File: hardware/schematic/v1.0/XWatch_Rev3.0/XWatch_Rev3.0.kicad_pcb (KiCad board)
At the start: 2 copper layers, 36 x 36 mm, 158 parts, among them CN1 SCTA1A0100, CN2 SCTA1A0100, CN3 SCTA1A0100, CN4 SCTA1A0100, CN5 SCTA1A0100, CN6 SCTA1A0100, IC1 nRF52833-QDAA-R, U10 OPT3001DNPR, U11 MAX30101EFD_T, U12 DRV2605LDGSR, U13 SK6018D4-33, U14 AXE530127-DO0143FMST02, U15 STM32U5A9BJY6QTR, U16 R832000033-32MHZ, U2 GD25LQ128EWIGR, U3 DA9168, U4 TPS62840DLCR, U5 MAX17048G_T10, U6 LSM6DSOXTR, U7 LIS2MDLTR, U8 SM03B-SRSS-TB_LF_SN_P, U9 LPS27HHWTR, X1 32.768KHZ, X2 16MHZ, X3 32.768KHZ

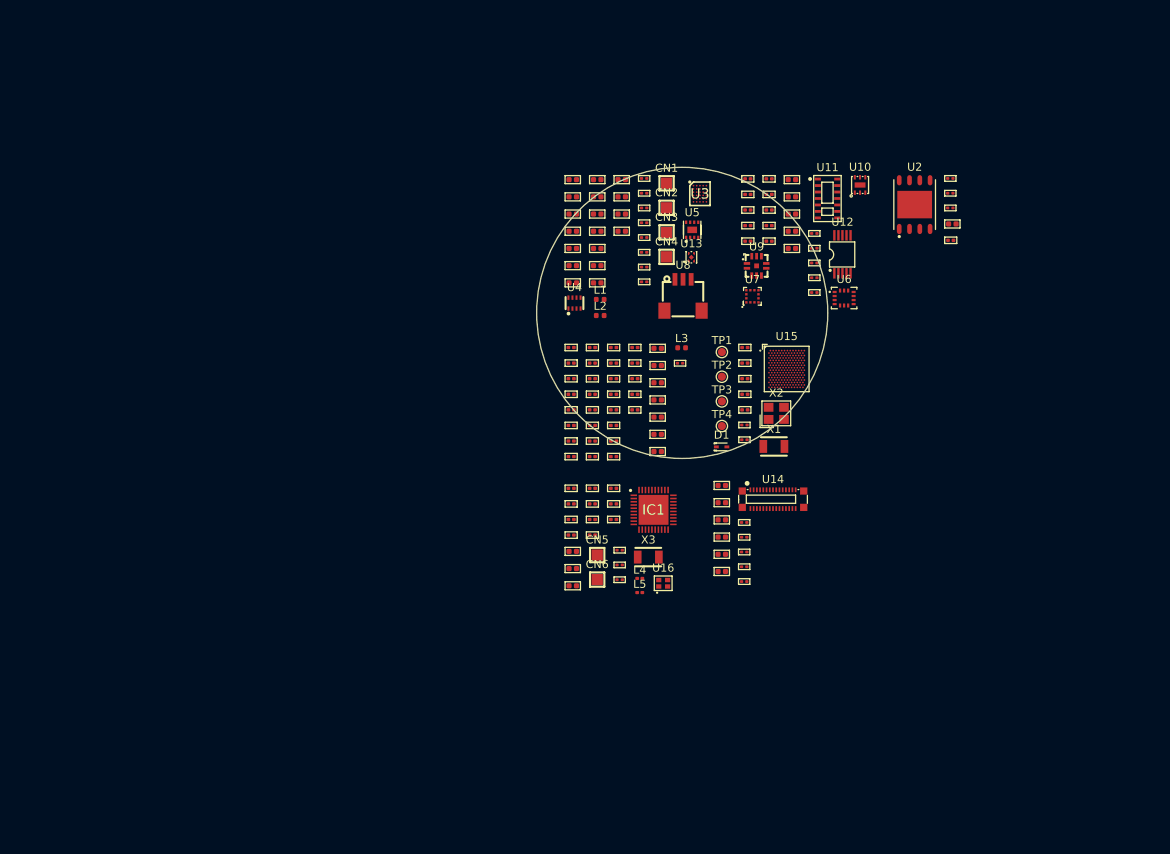
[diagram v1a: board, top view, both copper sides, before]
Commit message: add pdf
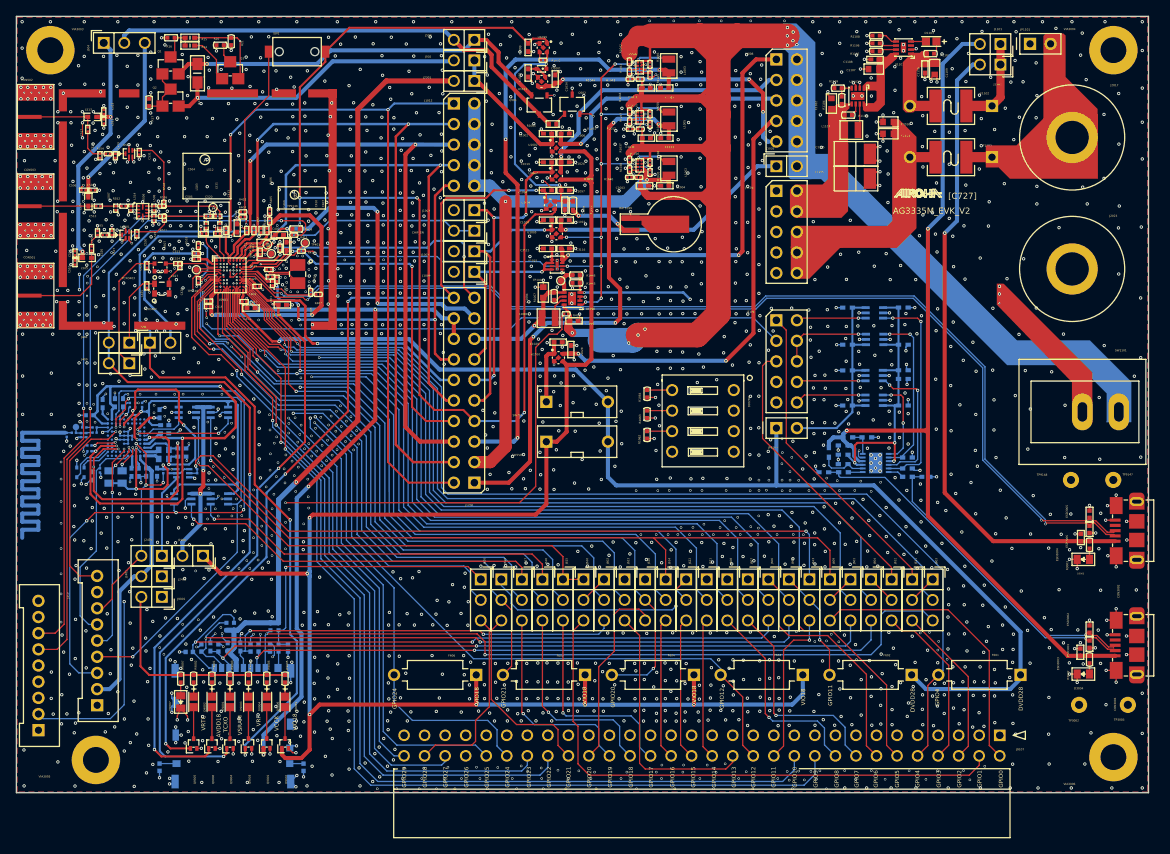
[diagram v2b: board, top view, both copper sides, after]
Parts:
- removed C1, C2, C86, C87: 5.6pF, XWatch_Rev3.0:GEN_C_0201
- removed C10, C109, C16, C17, C30, C59, C6, C63, C78, C9: 10uF, XWatch_Rev3.0:GEN_C_0402
- removed C100, C103, C106, C107, C108, C110, C111, C112, C113, C20, C21, C22, C23, C24, C25, C26, C27, C28, C29, C48, C50, C51, C53, C54, C55, C56, C57, C58, C60, C67, C69, C70, C72, C79, C89, C90, C91, C92, C93, C94, C95, C96, C97, C98: 100nF, XWatch_Rev3.0:GEN_C_0201
- removed C101, C102, C18, C19, C61, C62, C64, C65, C66, C68, C74, C76, C80, C81: 1uF, XWatch_Rev3.0:GEN_C_0402
- removed C104, C105, C11, C12, C13: 2.2uF, XWatch_Rev3.0:GEN_C_0402
- removed C14, C49, C7, C73, C75, C77: 100nF, XWatch_Rev3.0:GEN_C_0402
- removed C15, C5, C71, C99: 4.7uF, XWatch_Rev3.0:GEN_C_0402
- removed C3, C4: 10pF, XWatch_Rev3.0:GEN_C_0201
- removed C52: 220nF, XWatch_Rev3.0:GEN_C_0201
- removed C8: 47nF, XWatch_Rev3.0:GEN_C_0402
- removed C82: 1pF, XWatch_Rev3.0:GEN_C_0201
- removed C83: 1.2pF, XWatch_Rev3.0:GEN_C_0201
- removed C84, C85: 12pF, XWatch_Rev3.0:GEN_C_0201
- removed C88: 100pF, XWatch_Rev3.0:GEN_C_0201
- removed CN1, CN2, CN3, CN4, CN5, CN6: SCTA1A0100, XWatch_Rev3.0:SCTA1A0100
- removed D1: RB520S-30, XWatch_Rev3.0:RB520S-30_C7502701
- removed IC1: nRF52833-QDAA-R, XWatch_Rev3.0:QFN40P500X500X90-41N
- removed L1, L2, L3: 2.2uH, XWatch_Rev3.0:L_0402_1005Metric
- removed L4: 4.7nH, XWatch_Rev3.0:L_0201_0603Metric
- removed L5: 2.2nH, XWatch_Rev3.0:L_0201_0603Metric
- removed R10: 38.3 k 1%, XWatch_Rev3.0:GEN_R_0201
- removed R11, R12: 2.2K, XWatch_Rev3.0:GEN_R_0201
- removed R18, R23, R24, R25, R6, R7, R8: 10K, XWatch_Rev3.0:GEN_R_0201
- removed R19, R26, R27, R28, R3: 100K, XWatch_Rev3.0:GEN_R_0201
- removed R22, R29: 0, XWatch_Rev3.0:GEN_R_0201
- removed R4, R5: 4.7K, XWatch_Rev3.0:GEN_R_0201
- removed R9: 24.9 k 1%, XWatch_Rev3.0:GEN_R_0201
- removed TP1, TP2, TP3, TP4: TestPoint, TestPoint:TestPoint_Pad_D1.0mm
- removed U10: OPT3001DNPR, XWatch_Rev3.0:OPT3001DNPR
- removed U11: MAX30101EFD_T, XWatch_Rev3.0:MAX30101EFD_T
- removed U12: DRV2605LDGSR, XWatch_Rev3.0:DRV2605LDGSR
- removed U13: SK6018D4-33, XWatch_Rev3.0:SK6018D4-33
- removed U14: AXE530127-DO0143FMST02, XWatch_Rev3.0:AXE530127
- removed U15: STM32U5A9BJY6QTR, XWatch_Rev3.0:STM32U5A9BJY6QTR
- removed U16: R832000033-32MHZ, XWatch_Rev3.0:R832000033
- removed U2: GD25LQ128EWIGR, XWatch_Rev3.0:GD25LQ128EWIGR
- removed U3: DA9168, XWatch_Rev3.0:BGA30C40P5X6_214X254X56
- removed U4: TPS62840DLCR, XWatch_Rev3.0:TPS62840DLCR
- removed U5: MAX17048G_T10, XWatch_Rev3.0:MAX17048G_T10
- removed U6: LSM6DSOXTR, XWatch_Rev3.0:LSM6DSOXTR
- removed U7: LIS2MDLTR, XWatch_Rev3.0:LIS2MDLTR
- removed U8: SM03B-SRSS-TB_LF_SN_P, XWatch_Rev3.0:SM03B-SRSS-TB_LF_SN_P
- removed U9: LPS27HHWTR, XWatch_Rev3.0:LPS27HHWTR
- removed X1, X3: 32.768KHZ, XWatch_Rev3.0:NX3215SA_32_768KHZ_EXS00A-MU00525
- removed X2: 16MHZ, XWatch_Rev3.0:TXM16M0004252CBCEO00T
- added BAT1099: C0.22F3.3V$2F$SMD$2F$EN-RL, C0.22F3.3V$2F$SMD$2F$EN-RL, F.Cu at (154.7, 82.7)
- added C0401: C0201, C0201, F.Cu at (110.7, 89.5)
- added C0501: C0201, C0201, F.Cu at (87.8, 85.7)
- added C1002: C0402, C0402, F.Cu at (144.2, 71.5)
- added C1003: C0402, C0402, F.Cu at (156.2, 78.0)
- added C1004: C0402, C0402, F.Cu at (158.7, 78.0)
- added C1006: C0402, C0402, F.Cu at (146.4, 71.5)
- added C1014: C0402, C0402, F.Cu at (144.2, 82.2)
- added C1015: C0402, C0402, F.Cu at (146.4, 82.2)
- added C1019: C0402, C0402, F.Cu at (144.2, 75.0)
- added C1021: C0402, C0402, F.Cu at (156.4, 65.9)
- added C1022: C0402, C0402, F.Cu at (158.7, 65.9)
- added C1024: C0402, C0402, F.Cu at (146.4, 75.0)
- added C1025: C0402, C0402, F.Cu at (145.5, 97.3)
- added C1028: C0402, C0402, F.Cu at (147.1, 98.2)
- added C1030: C0402, C0402, F.Cu at (156.4, 72.1)
- added C1031: C0402, C0402, F.Cu at (158.7, 72.1)
- added C1034: C0402, C0402, F.Cu at (145.1, 64.7)
- added C1035: C0402, C0402, F.Cu at (141.8, 64.0)
- added C1094: C0603, C0603, F.Cu at (143.7, 91.1)
- added C1095: C0402, C0402, F.Cu at (147.5, 94.7)
- added C1096: C0402, C0402, F.Cu at (144.2, 78.5)
- added C1097: C0402, C0402, F.Cu at (146.4, 78.5)
- added C1098: C0402, C0402, F.Cu at (146.3, 80.4)
- added C1099: C0402, C0402, F.Cu at (141.8, 60.8)
- added C1102: C0603, C0603, F.Cu at (179.3, 67.8)
- added C1104: C0603, C0603, F.Cu at (186.3, 71.5)
- added C1105: C1210, C1210, F.Cu at (182.3, 74.0)
- added C1106: C1210, C1210, F.Cu at (182.3, 77.1)
- added C1107: C0603, C0603, F.Cu at (184.5, 63.5)
- added C1108: C0402, C0402, F.Cu at (184.7, 62.3)
- added C1109: C0603, C0603, F.Cu at (192.1, 63.5)
- added C1110: C0402, C0402, F.Cu at (190.8, 63.5)
- added C2016: C0603, C0603, F.Cu at (186.3, 70.1)
- added C2301: C0402, C0402, B.Cu at (104.6, 135.0)
- added C2302: C0402, C0402, B.Cu at (106.2, 135.0)
- added C2303: C0402, C0402, B.Cu at (102.5, 135.0)
- added C2401: C0201, C0201, B.Cu at (87.2, 108.8)
- added C2402: C0402, C0402, B.Cu at (99.0, 110.4)
- added C2403: C0402, C0402, B.Cu at (96.8, 107.6)
- added C2404: C0402, C0402, B.Cu at (96.8, 108.6)
- added C2405: C0201, C0201, B.Cu at (87.5, 110.1)
- added C2406: C0201, C0201, B.Cu at (87.5, 110.8)
- added C2407: C0402, C0402, B.Cu at (95.9, 113.4)
- added C2408: C0201, C0201, B.Cu at (84.7, 108.7)
- added C2409: C0201, C0201, B.Cu at (86.5, 108.8)
- added C2410: C0201, C0201, B.Cu at (86.9, 107.8)
- added C2411: C0402, C0402, B.Cu at (87.9, 113.8)
- added C2412: C0402, C0402, B.Cu at (94.6, 113.4)
- added C2413: C0402, C0402, B.Cu at (99.0, 111.4)
- added C2414: C0402, C0402, B.Cu at (93.6, 113.4)
- added C2415: C0402, C0402, B.Cu at (96.2, 106.1)
- added C2416: C0402, C0402, B.Cu at (92.7, 113.4)
- added C2417: C0402, C0402, B.Cu at (87.5, 106.3)
- added C2418: C0201, C0201, B.Cu at (93.2, 105.1)
- added C2419: C0402, C0402, B.Cu at (89.2, 104.9)
- added C2420: C0402, C0402, B.Cu at (90.7, 104.8)
- added C2421: C0201, C0201, B.Cu at (94.0, 105.1)
- added C3101: SC0402, SC0402, B.Cu at (180.7, 112.4)
- added C3102: C0402, C0402, B.Cu at (191.0, 113.9)
- added C3103: SC0402, SC0402, B.Cu at (188.2, 100.8)
- added C3104: SC0402, SC0402, B.Cu at (181.3, 100.8)
- added C3105: SC0402, SC0402, B.Cu at (178.3, 113.4)
- added C3106: SC0402, SC0402, B.Cu at (188.2, 97.6)
- added C3107: SC0402, SC0402, B.Cu at (180.7, 110.1)
- added C3108: SC0402, SC0402, B.Cu at (180.7, 111.2)
- added C3109: SC0402, SC0402, B.Cu at (188.2, 93.0)
- added C3110: SC0402, SC0402, B.Cu at (181.3, 93.0)
- added C3111: SC0402, SC0402, B.Cu at (188.2, 105.1)
- added C3112: SC0402, SC0402, B.Cu at (181.3, 97.6)
- added C3113: SC0402, SC0402, B.Cu at (188.2, 101.8)
- added C3114: SC0402, SC0402, B.Cu at (181.3, 105.1)
- added C3115: C0402, C0402, F.Cu at (144.2, 85.7)
- added C3116: C0402, C0402, F.Cu at (146.4, 85.7)
- added C402: C0201, C0201, F.Cu at (108.8, 83.5)
- added C403: C0201, C0201, F.Cu at (109.5, 83.5)
- added C404: C0402, C0402, F.Cu at (105.8, 83.2)
- added C405: C0402, C0402, F.Cu at (111.0, 84.0)
- added C406: C0402, C0402, F.Cu at (111.4, 92.7)
- added C407: C0201, C0201, F.Cu at (111.1, 85.7)
- added C408: C0201, C0201, F.Cu at (108.3, 90.4)
- added C409: C0201, C0201, F.Cu at (108.7, 86.2)
- added C410: C0402, C0402, F.Cu at (111.9, 85.4)
- added C411: C0201, C0201, F.Cu at (107.0, 83.5)
- added C412: C0201, C0201, F.Cu at (107.9, 83.5)
- added C413: C0201, C0201, F.Cu at (104.4, 83.5)
- added C414: C0402, C0402, F.Cu at (107.5, 93.1)
- added C415: C0201, C0201, F.Cu at (102.3, 92.9)
- added C416: C0201, C0201, F.Cu at (102.3, 92.2)
- added C417: C0201, C0201, F.Cu at (106.7, 92.3)
- added C419: C0201, C0201, F.Cu at (109.7, 88.3)
- added C420: C0201, C0201, F.Cu at (109.9, 89.2)
- added C425: C0201, C0201, F.Cu at (94.6, 90.3)
- added C426: C0201, C0201, F.Cu at (98.7, 87.8)
- added C427: C0201, C0201, F.Cu at (98.5, 87.6)
- added C428: C0201, C0201, F.Cu at (94.6, 87.8)
- added C504: C0201, C0201, F.Cu at (102.2, 81.7)
- added C505: C0201, C0201, F.Cu at (101.7, 83.9)
- added C506: C0201, C0201, F.Cu at (86.8, 78.5)
- added C508: C0201, C0201, F.Cu at (88.0, 78.5)
- added C510: C0201, C0201, F.Cu at (85.7, 87.5)
- added C511: C0201, C0201, F.Cu at (85.7, 86.3)
- added C513: C0201, C0201, F.Cu at (88.6, 80.5)
- added C517: C0201, C0201, F.Cu at (87.3, 71.0)
- added C520: C0201, C0201, F.Cu at (103.4, 83.9)
- added C521: C0201, C0201, F.Cu at (89.3, 70.0)
- added C522: C0201, C0201, F.Cu at (89.3, 68.8)
- added C523: C0201, C0201, F.Cu at (100.8, 86.3)
- added C524: C0201, C0201, F.Cu at (100.8, 87.0)
- added C525: C0201, C0201, F.Cu at (101.0, 89.7)
- added C526: C0201, C0201, F.Cu at (88.5, 83.8)
- added C527: C0201, C0201, F.Cu at (90.3, 83.8)
- added C528: C0201, C0201, F.Cu at (88.8, 74.2)
- added C529: C0201, C0201, F.Cu at (90.7, 74.2)
- added C530: C0201, C0201, F.Cu at (93.4, 83.9)
- added C531: C0201, C0201, F.Cu at (93.7, 73.8)
- added CHIP_EN: DIP2$2F$P2.54, DIP2$2F$P2.54, F.Cu at (135.1, 83.5)
- added CON2301: MICROSD$2F$8P$2F$SMD$2F$TA-M017-012-07-811, MICROSD$2F$8P$2F$SMD$2F$TA-M017-012-07-811, B.Cu at (103.0, 137.1)
- added CON3001: MICROUSB$2F$5P$2F$SMD$2F$P0.65$2F$R$2F$8791-N005-M1A0, MICROUSB$2F$5P$2F$SMD$2F$P0.65$2F$R$2F$8791-N005-M1A0, F.Cu at (214.4, 134.8)
- added CON3002: MICROUSB$2F$5P$2F$SMD$2F$P0.65$2F$R$2F$8791-N005-M1A0, MICROUSB$2F$5P$2F$SMD$2F$P0.65$2F$R$2F$8791-N005-M1A0, F.Cu at (214.4, 120.6)
- added CON501: SMA8400M, SMA8400M, F.Cu at (80.1, 91.5)
- added CON502: SMA8400M, SMA8400M, F.Cu at (80.1, 69.4)
- added CON503: SMA8400M, SMA8400M, F.Cu at (80.1, 80.5)
- added D1001: D$2F$SMD$2F$VMD2, D$2F$SMD$2F$VMD2, F.Cu at (143.4, 63.5)
- added D1103: LED190, LED190, F.Cu at (191.6, 60.1)
- added D2401: LED-S, LED-S, B.Cu at (91.6, 114.0)
- added D2402: LED-S, LED-S, B.Cu at (90.0, 114.0)
- added D3004: LED-S, LED-S, F.Cu at (210.4, 138.3)
- added D3005: LED-S, LED-S, F.Cu at (210.4, 124.1)
- added D9001: LED190, LED190, F.Cu at (102.7, 141.8)
- added D9002: LED190, LED190, F.Cu at (100.4, 141.8)
- added D9003: LED190, LED190, F.Cu at (104.9, 141.8)
- added D9004: LED190, LED190, F.Cu at (107.2, 141.8)
- added D9005: LED190, LED190, F.Cu at (111.7, 141.8)
- added D9006: LED190, LED190, F.Cu at (109.5, 141.8)
- added D9007: LED-S, LED-S, F.Cu at (98.8, 141.8)
- added ESD2301: VR0402, VR0402, B.Cu at (112.1, 135.1)
- added ESD2302: VR0402, VR0402, B.Cu at (109.9, 135.1)
- added ESD2303: VR0402, VR0402, B.Cu at (108.4, 135.1)
- added ESD2304: VR0402, VR0402, B.Cu at (107.5, 135.1)
- added ESD2305: VR0402, VR0402, B.Cu at (103.5, 135.1)
- added ESD2306: VR0402, VR0402, B.Cu at (101.4, 135.1)
- added ESD2307: VR0402, VR0402, B.Cu at (99.9, 135.6)
- added ESD2308: VR0402, VR0402, B.Cu at (114.0, 149.9)
- added ESD239: VR0402, VR0402, B.Cu at (96.2, 149.9)
- added ESD3001: VR0402, VR0402, F.Cu at (211.2, 134.6)
- added ESD3002: VR0402, VR0402, F.Cu at (211.2, 132.8)
- added ESD3003: VR0402, VR0402, F.Cu at (210.1, 135.6)
- added ESD3004: VR0402, VR0402, F.Cu at (210.1, 121.5)
- added ESD3005: VR0402, VR0402, F.Cu at (211.2, 118.6)
- added ESD3006: VR0402, VR0402, F.Cu at (211.2, 120.4)
- added F1102: FUSE$2F$DIP$2F$SMD, FUSE$2F$DIP$2F$SMD, F.Cu at (199.2, 68.1)
- added F1103: FUSE$2F$DIP$2F$SMD, FUSE$2F$DIP$2F$SMD, F.Cu at (199.2, 74.4)
- added F601: R$5C$DIP, R$5C$DIP, F.Cu at (197.6, 138.4)
- added F602: R$5C$DIP, R$5C$DIP, F.Cu at (184.1, 138.4)
- added F603: R$5C$DIP, R$5C$DIP, F.Cu at (170.7, 138.4)
- added F604: R$5C$DIP, R$5C$DIP, F.Cu at (157.2, 138.4)
- added F605: R$5C$DIP, R$5C$DIP, F.Cu at (143.7, 138.4)
- added F606: R$5C$DIP, R$5C$DIP, F.Cu at (130.3, 138.4)
- added J1002: DIP2$2F$P2.54, DIP2$2F$P2.54, F.Cu at (135.1, 81.0)
- added J1005: DIP2$2F$P2.54, DIP2$2F$P2.54, F.Cu at (172.5, 75.5)
- added J1007: DIP2$2F$P2.54, DIP2$2F$P2.54, F.Cu at (135.1, 86.1)
- added J1008: HEADER10, HEADER10, F.Cu at (172.5, 62.3)
- added J1009: DIP2$2F$P2.54, DIP2$2F$P2.54, F.Cu at (135.1, 88.6)
- added J1012: HEADER10, HEADER10, F.Cu at (132.6, 67.8)
- added J1101: DIP2$2F$P2.54, DIP2$2F$P2.54, F.Cu at (200.2, 60.4)
- added J1102: DIP2$2F$P2.54, DIP2$2F$P2.54, F.Cu at (200.2, 63.0)
- added J1103: HEADER10, HEADER10, F.Cu at (172.5, 78.6)
- added J1206: HEADER10X2-P2.54, HEADER10X2-P2.54, F.Cu at (132.6, 91.8)
- added J2017: JACK$2F$BANAAA, JACK$2F$BANAAA, F.Cu at (209.1, 72.0)
- added J2023: JACK$2F$BANAAA, JACK$2F$BANAAA, F.Cu at (209.1, 88.2)
- added J2301: DIP2$2F$P2.54, DIP2$2F$P2.54, F.Cu at (135.1, 65.0)
- added J2401: SIP-9P-2MM-FRAME, SIP-9P-2MM-FRAME, F.Cu at (88.5, 134.2)
- added J2402: DIP2$2F$P2.54, DIP2$2F$P2.54, F.Cu at (96.5, 126.3)
- added J2403: DIP2$2F$P2.54, DIP2$2F$P2.54, F.Cu at (96.5, 123.7)
- added J3101: HEADER10, HEADER10, F.Cu at (172.5, 94.6)
- added J408: DIP2$2F$P2.54, DIP2$2F$P2.54, F.Cu at (92.5, 97.4)
- added J409: DIP2$2F$P2.54, DIP2$2F$P2.54, F.Cu at (92.5, 99.9)
- added J412: SIP-9P-2MM-FRAME, SIP-9P-2MM-FRAME, F.Cu at (81.2, 137.3)
- added J501: DIP2$2F$P2.54, DIP2$2F$P2.54, F.Cu at (95.0, 97.4)
- added J502: DIP2$2F$P2.54, DIP2$2F$P2.54, F.Cu at (135.1, 62.4)
- added J503: DIP2$2F$P2.54, DIP2$2F$P2.54, F.Cu at (135.1, 59.9)
- added J504: DIP3$2F$P2.54, DIP3$2F$P2.54, F.Cu at (89.3, 60.3)
- added J601: DIP3$2F$P2.54, DIP3$2F$P2.54, F.Cu at (181.7, 126.6)
- added J602: DIP3$2F$P2.54, DIP3$2F$P2.54, F.Cu at (151.2, 126.6)
- added J603: DIP3$2F$P2.54, DIP3$2F$P2.54, F.Cu at (191.8, 126.6)
- added J604: DIP3$2F$P2.54, DIP3$2F$P2.54, F.Cu at (184.2, 126.6)
- added J605: DIP3$2F$P2.54, DIP3$2F$P2.54, F.Cu at (174.0, 126.6)
- added J606: DIP3$2F$P2.54, DIP3$2F$P2.54, F.Cu at (171.5, 126.6)
- added J607: DIP3$2F$P2.54, DIP3$2F$P2.54, F.Cu at (169.0, 126.6)
- added J608: DIP3$2F$P2.54, DIP3$2F$P2.54, F.Cu at (166.4, 126.6)
- added J609: DIP3$2F$P2.54, DIP3$2F$P2.54, F.Cu at (179.1, 126.6)
- added J610: DIP3$2F$P2.54, DIP3$2F$P2.54, F.Cu at (148.6, 126.6)
- added J611: DIP3$2F$P2.54, DIP3$2F$P2.54, F.Cu at (189.3, 126.6)
- added J612: DIP3$2F$P2.54, DIP3$2F$P2.54, F.Cu at (186.7, 126.6)
- added J613: DIP3$2F$P2.54, DIP3$2F$P2.54, F.Cu at (176.6, 126.6)
- added J614: DIP3$2F$P2.54, DIP3$2F$P2.54, F.Cu at (158.8, 126.6)
- added J615: DIP3$2F$P2.54, DIP3$2F$P2.54, F.Cu at (146.1, 126.6)
- added J616: DIP3$2F$P2.54, DIP3$2F$P2.54, F.Cu at (143.6, 126.6)
- added J617: DIP3$2F$P2.54, DIP3$2F$P2.54, F.Cu at (141.0, 126.6)
- added J618: DIP3$2F$P2.54, DIP3$2F$P2.54, F.Cu at (156.3, 126.6)
- added J619: DIP3$2F$P2.54, DIP3$2F$P2.54, F.Cu at (138.5, 126.6)
- added J620: DIP3$2F$P2.54, DIP3$2F$P2.54, F.Cu at (135.9, 126.6)
- added J621: DIP3$2F$P2.54, DIP3$2F$P2.54, F.Cu at (163.9, 126.6)
- added J622: DIP3$2F$P2.54, DIP3$2F$P2.54, F.Cu at (161.3, 126.6)
- added J623: DIP3$2F$P2.54, DIP3$2F$P2.54, F.Cu at (153.7, 126.6)
- added J9001: DIP2$2F$P2.54, DIP2$2F$P2.54, F.Cu at (96.5, 128.8)
- added J9107: DIP30X2$2F$P2.54$2F$R$2F$PHR230GB138, DIP30X2$2F$P2.54$2F$R$2F$PHR230GB138, F.Cu at (200.1, 145.9)
- added J9109: DIP2$2F$P2.54, DIP2$2F$P2.54, F.Cu at (101.6, 123.7)
- added JP1101: SIP-2P, SIP-2P, F.Cu at (203.9, 60.4)
- added JP3103: SIP-2P, SIP-2P, F.Cu at (172.5, 107.9)
- added L1001: L$2F$IND$2F$SMD$2F$2520, L$2F$IND$2F$SMD$2F$2520, F.Cu at (144.3, 94.3)
- added L1002: L$2F$IND$2F$SMD$2F$LQM2MP-0806, L$2F$IND$2F$SMD$2F$LQM2MP-0806, F.Cu at (159.2, 75.8)
- added L1003: L$2F$IND$2F$SMD$2F$LQM2MP-0806, L$2F$IND$2F$SMD$2F$LQM2MP-0806, F.Cu at (159.2, 63.1)
- added L1005: L$2F$IND$2F$SMD$2F$LQM2MP-0806, L$2F$IND$2F$SMD$2F$LQM2MP-0806, F.Cu at (159.2, 69.7)
- added L1102: L$2F$IND$2F$SMD$2F$2520, L$2F$IND$2F$SMD$2F$2520, F.Cu at (181.8, 71.1)
- added L2401: C0201, C0201, B.Cu at (88.2, 108.5)
- added L2402: C0603_H300, C0603_H300, B.Cu at (96.7, 110.8)
- added L2403: C0201, C0201, B.Cu at (88.2, 107.8)
- added L2404: C0603_H300, C0603_H300, B.Cu at (96.7, 111.9)
- added L401: L0201, L0201, F.Cu at (110.2, 90.0)
- added L503: L0201, L0201, F.Cu at (102.0, 82.9)
- added L504: L$2F$IND$2F$SMD$2F$0402, L$2F$IND$2F$SMD$2F$0402, F.Cu at (87.4, 79.9)
- added L505: L$2F$IND$2F$SMD$2F$0402, L$2F$IND$2F$SMD$2F$0402, F.Cu at (87.2, 86.9)
- added L507: L0201, L0201, F.Cu at (90.8, 80.7)
- added L508: L0201, L0201, F.Cu at (95.5, 80.7)
- added L511: L0201, L0201, F.Cu at (103.7, 82.9)
- added L512: L0201, L0201, F.Cu at (103.4, 81.7)
- added L513: L$2F$IND$2F$SMD$2F$0402, L$2F$IND$2F$SMD$2F$0402, F.Cu at (87.9, 69.4)
- added L514: L0201, L0201, F.Cu at (92.7, 80.7)
- added L515: L0201, L0201, F.Cu at (95.5, 82.0)
- added PF_TEST2401: PADCB, PADCB, B.Cu at (85.6, 107.8)
- added Q1: SOT-23, SOT-23, F.Cu at (96.6, 64.1)
- added Q2: SOT-23, SOT-23, F.Cu at (96.6, 68.1)
- added Q3: SOT-23, SOT-23, F.Cu at (103.9, 64.7)
- added Q501: SPP2301_USI, SPP2301_USI, F.Cu at (143.2, 68.0)
- added Q502: SPP2301_USI, SPP2301_USI, F.Cu at (147.2, 67.9)
- added Q9001: 2-1L1B$2F$SMD$2F$SSM3K35MFV, 2-1L1B$2F$SMD$2F$SSM3K35MFV, F.Cu at (109.5, 146.9)
- added Q9002: 2-1L1B$2F$SMD$2F$SSM3K35MFV, 2-1L1B$2F$SMD$2F$SSM3K35MFV, F.Cu at (111.7, 146.9)
- added Q9003: 2-1L1B$2F$SMD$2F$SSM3K35MFV, 2-1L1B$2F$SMD$2F$SSM3K35MFV, F.Cu at (107.2, 146.9)
- added Q9004: 2-1L1B$2F$SMD$2F$SSM3K35MFV, 2-1L1B$2F$SMD$2F$SSM3K35MFV, F.Cu at (104.9, 146.9)
- added Q9005: 2-1L1B$2F$SMD$2F$SSM3K35MFV, 2-1L1B$2F$SMD$2F$SSM3K35MFV, F.Cu at (100.4, 146.9)
- added Q9006: 2-1L1B$2F$SMD$2F$SSM3K35MFV, 2-1L1B$2F$SMD$2F$SSM3K35MFV, F.Cu at (102.7, 146.9)
- added R1033: R0201, R0201, F.Cu at (143.6, 62.4)
- added R1035: R0201, R0201, F.Cu at (156.9, 76.3)
- added R1036: R0201, R0201, F.Cu at (156.9, 75.1)
- added R1037: R0201, R0201, F.Cu at (154.3, 74.8)
- added R1038: R0201, R0201, F.Cu at (154.3, 76.0)
- added R1039: R0201, R0201, F.Cu at (154.3, 76.9)
- added R1040: R0201, R0201, F.Cu at (155.5, 76.9)
- added R1041: R0201, R0201, F.Cu at (154.3, 63.9)
- added R1042: R0201, R0201, F.Cu at (154.3, 62.6)
- added R1043: R0201, R0201, F.Cu at (155.6, 64.8)
- added R1044: R0201, R0201, F.Cu at (154.4, 64.8)
- added R1045: R0201, R0201, F.Cu at (156.9, 64.3)
- added R1046: R0201, R0201, F.Cu at (156.9, 62.9)
- added R1047: R0201, R0201, F.Cu at (154.3, 70.0)
- added R1048: R0201, R0201, F.Cu at (154.3, 68.8)
- added R1049: R0201, R0201, F.Cu at (156.9, 70.4)
- added R1050: R0201, R0201, F.Cu at (156.9, 69.1)
- added R1051: R0201, R0201, F.Cu at (154.4, 70.9)
- added R1052: R0201, R0201, F.Cu at (155.6, 70.9)
- added R1060: R0402$2F$SMD, R0402$2F$SMD, F.Cu at (147.3, 80.4)
- added R1061: 0402_USI, 0402_USI, F.Cu at (144.8, 70.3)
- added R1062: R0402, R0402, F.Cu at (156.5, 108.8)
- added R1063: R0402, R0402, F.Cu at (156.5, 106.2)
- added R1064: R0402, R0402, F.Cu at (156.5, 103.7)
- added R1065: R0402, R0402, F.Cu at (147.7, 90.0)
- added R1067: R0402, R0402, F.Cu at (145.0, 91.6)
- added R1068: R0402, R0402, F.Cu at (147.7, 89.0)
- added R1103: R0402, R0402, F.Cu at (191.5, 61.6)
- added R1104: R0402, R0402, F.Cu at (180.6, 67.4)
- added R1105: R0402, R0402, F.Cu at (181.4, 69.2)
- added R1106: R0402, R0402, F.Cu at (184.8, 60.3)
- added R1107: R0402, R0402, F.Cu at (184.8, 61.3)
- added R1108: R0402, R0402, F.Cu at (184.8, 59.4)
- added R1109: R0402, R0402, F.Cu at (180.1, 65.9)
- added R2308: R0402, R0402, B.Cu at (109.9, 132.5)
- added R2309: R0402, R0402, B.Cu at (105.4, 132.5)
- added R2310: R0402, R0402, B.Cu at (104.5, 132.5)
- added R2311: R0402, R0402, B.Cu at (110.9, 132.5)
- added R2312: R0402, R0402, B.Cu at (110.9, 135.1)
- added R2401: R0201, R0201, B.Cu at (85.6, 108.5)
- added R2402: C0201, C0201, B.Cu at (92.5, 105.1)
- added R2403: C0402, C0402, B.Cu at (91.7, 104.8)
- added R2404: C0201, C0201, B.Cu at (88.8, 113.1)
- added R2405: R0201, R0201, B.Cu at (97.3, 113.2)
- added R2406: R0201, R0201, B.Cu at (96.7, 113.2)
- added R2409: R0201, R0201, B.Cu at (100.9, 113.2)
- added R3002: R0402, R0402, F.Cu at (211.2, 136.5)
- added R3003: R0402, R0402, F.Cu at (211.2, 122.4)
- added R3101: SR0402, SR0402, B.Cu at (179.0, 110.9)
- added R3102: SR0402, SR0402, B.Cu at (188.7, 113.9)
- added R3103: SR0402, SR0402, B.Cu at (181.3, 109.1)
- added R3104: SR0402, SR0402, B.Cu at (188.7, 112.9)
- added R3105: SR0402, SR0402, B.Cu at (180.8, 113.4)
- added R3106: SR0402, SR0402, B.Cu at (188.7, 111.6)
- added R3107: SR0402, SR0402, B.Cu at (183.7, 109.1)
- added R404: R0201, R0201, F.Cu at (106.5, 81.8)
- added R405: R0201, R0201, F.Cu at (109.8, 82.3)
- added R406: R0201, R0201, F.Cu at (109.8, 81.1)
- added R407: R0201, R0201, F.Cu at (115.8, 91.4)
- added R408: R0201, R0201, F.Cu at (114.9, 91.1)
- added R409: R0402, R0402, F.Cu at (113.1, 83.3)
- added R410: R0201, R0201, F.Cu at (146.5, 93.8)
- added R411: R0201, R0201, F.Cu at (112.8, 84.1)
- added R412: R0201, R0201, F.Cu at (106.5, 81.2)
- added R413: R0201, R0201, F.Cu at (113.7, 86.0)
- added R507: R0201, R0201, F.Cu at (96.8, 82.0)
- added R511: R0201, R0201, F.Cu at (96.5, 81.7)
- added R526: R0201, R0201, F.Cu at (96.5, 80.5)
- added R528: R0201, R0201, F.Cu at (96.7, 80.2)
- added R552: R0201, R0201, F.Cu at (91.8, 80.5)
- added R553: R0201, R0201, F.Cu at (101.0, 85.3)
- added R554: R0201, R0201, F.Cu at (89.8, 74.0)
- added R555: R0201, R0201, F.Cu at (89.4, 84.0)
- added R9001: R0402, R0402, F.Cu at (102.7, 138.9)
- added R9002: R0402, R0402, F.Cu at (100.4, 138.9)
- added R9003: R0402, R0402, F.Cu at (104.9, 138.9)
- added R9004: R0402, R0402, F.Cu at (107.2, 138.9)
- added R9005: R0402, R0402, F.Cu at (111.7, 138.9)
- added R9006: R0402, R0402, F.Cu at (109.5, 138.9)
- added R9007: R0402, R0402, F.Cu at (98.8, 138.9)
- added SHORT402: NC$2F$MMD$2F$L1$2F$4MIL, NC$2F$MMD$2F$L1$2F$4MIL, F.Cu at (108.8, 86.3)
- added SW1: TS6301E180G, TS6301E180G, F.Cu at (113.2, 61.4)
- added SW1101: SW2P$2F$DIP-V1, SW2P$2F$DIP-V1, F.Cu at (210.3, 105.9)
- added SW1V8: DIP-SWITCH_2X1, DIP-SWITCH_2X1, F.Cu at (144.0, 109.6)
- added SW2002: SW8P_DIP_P2.54, SW8P_DIP_P2.54, F.Cu at (163.4, 107.0)
- added SW2V8: DIP-SWITCH_2X1, DIP-SWITCH_2X1, F.Cu at (144.0, 104.7)
- added TCXO402: TXCO4P$2F$SMD$2F$P0.4$2F$2.0X1.6$2F$KT2016K, TXCO4P$2F$SMD$2F$P0.4$2F$2.0X1.6$2F$KT2016K, F.Cu at (96.5, 90.7)
- added TCXO403: TXCO4P$2F$SMD$2F$P0.4$2F$1.65X1.25$2F$1612TCXO, TXCO4P$2F$SMD$2F$P0.4$2F$1.65X1.25$2F$1612TCXO, F.Cu at (96.3, 88.0)
- added TP1001: TP30MIL, TP30MIL, F.Cu at (145.8, 89.7)
- added TP3002: HOLE$2F$PTH$2F$D1R2, HOLE$2F$PTH$2F$D1R2, F.Cu at (209.9, 142.1)
- added TP3003: HOLE$2F$PTH$2F$D1R2, HOLE$2F$PTH$2F$D1R2, F.Cu at (215.9, 142.1)
- added TP401: TP30MIL, TP30MIL, F.Cu at (114.2, 85.0)
- added TP9146: TP30MIL, TP30MIL, F.Cu at (110.0, 86.4)
- added TP9147: HOLE$2F$PTH$2F$D1R2, HOLE$2F$PTH$2F$D1R2, F.Cu at (214.1, 114.3)
- added TP9148: HOLE$2F$PTH$2F$D1R2, HOLE$2F$PTH$2F$D1R2, F.Cu at (208.9, 114.3)
- added TP9149: TP30MIL, TP30MIL, F.Cu at (100.8, 88.3)
- added U0401: AG3335M_3.8X4.2(R9XC10)-0.4BPAA, AG3335M_3.8X4.2(R9XC10)-0.4BPAA, F.Cu at (104.9, 89.0)
- added U0501: SAW-1.1X0.9, SAW-1.1X0.9, F.Cu at (92.0, 84.0)
- added U1002: ZQFN-4L-1X1, ZQFN-4L-1X1, F.Cu at (145.3, 73.3)
- added U1005: ZQFN-4L-1X1, ZQFN-4L-1X1, F.Cu at (145.3, 83.9)
- added U1007: ZQFN-4L-1X1, ZQFN-4L-1X1, F.Cu at (145.3, 76.7)
- added U1008: WL-CSP0.9X1.6-8, WL-CSP0.9X1.6-8, F.Cu at (155.6, 63.3)
- added U1010: ZQFN-4L-1X1, ZQFN-4L-1X1, F.Cu at (145.5, 99.2)
- added U1012: WL-CSP0.9X1.6-8, WL-CSP0.9X1.6-8, F.Cu at (155.6, 69.5)
- added U1014: ZQFN-4L-1X1, ZQFN-4L-1X1, F.Cu at (143.4, 65.1)
- added U1015: XDFN8-P0.4-1.6X1.2, XDFN8-P0.4-1.6X1.2, F.Cu at (145.4, 87.7)
- added U1016: WL-CSP0.9X1.6-8, WL-CSP0.9X1.6-8, F.Cu at (155.6, 75.4)
- added U1096: WDFN8$2F$SMD$2F$P0.5$2F$RT5715, WDFN8$2F$SMD$2F$P0.5$2F$RT5715, F.Cu at (147.2, 91.9)
- added U1098: ZQFN-4L-1X1, ZQFN-4L-1X1, F.Cu at (144.5, 80.3)
- added U1099: ZQFN-4L-1X1, ZQFN-4L-1X1, F.Cu at (143.7, 60.9)
- added U1101: WDFN8$2F$SMD$2F$P0.5$2F$RT9718, WDFN8$2F$SMD$2F$P0.5$2F$RT9718, F.Cu at (188.2, 60.9)
- added U1102: WDFN8$2F$SMD$2F$P0.5$2F$RT5715, WDFN8$2F$SMD$2F$P0.5$2F$RT5715, F.Cu at (182.5, 66.9)
- added U2401: SOT363-6PIN, SOT363-6PIN, B.Cu at (99.1, 116.7)
- added U2402: BGA76-5.5X5.5-AHT, BGA76-5.5X5.5-AHT, B.Cu at (92.1, 109.1)
- added U2403: SOT363-6PIN, SOT363-6PIN, B.Cu at (103.6, 116.7)
- added U2404: EMT6-P0.5, EMT6-P0.5, B.Cu at (99.1, 113.5)
- added U2405: SOT363-6PIN, SOT363-6PIN, B.Cu at (99.6, 106.0)
- added U2406: SOT363-6PIN, SOT363-6PIN, B.Cu at (103.6, 106.0)
- added U3101: DFN12, DFN12, B.Cu at (184.8, 112.2)
- added U3102: SOT363-6PIN, SOT363-6PIN, B.Cu at (184.6, 93.7)
- added U3103: SOT363-6PIN, SOT363-6PIN, B.Cu at (184.6, 97.0)
- added U3104: SOT363-6PIN, SOT363-6PIN, B.Cu at (184.6, 101.4)
- added U3105: SOT363-6PIN, SOT363-6PIN, B.Cu at (184.6, 104.5)
- added U506: SAW1511, SAW1511, F.Cu at (94.1, 81.1)
- added U509: SAW-1.1X0.9, SAW-1.1X0.9, F.Cu at (92.4, 74.0)
- added VIA3003: TH3MM, TH3MM, F.Cu at (82.7, 61.2)
- added VIA3004: TH3MM, TH3MM, F.Cu at (214.2, 61.2)
- added VIA3005: TH3MM, TH3MM, F.Cu at (88.3, 149.0)
- added VIA3006: TH3MM, TH3MM, F.Cu at (214.2, 148.6)
- added X0401: RTC3215, RTC3215, F.Cu at (113.3, 88.9)
- added Y2401: XT2016, XT2016, B.Cu at (85.6, 112.4)
- R13: value 4.7K -> R0805; footprint XWatch_Rev3.0:GEN_R_0201 -> R0805
- R14: value 4.7K -> SR0402; footprint XWatch_Rev3.0:GEN_R_0201 -> SR0402
- R15: value 10K -> SR0402; footprint XWatch_Rev3.0:GEN_R_0201 -> SR0402
- R16, R20, R21: value 10K -> R0402; footprint XWatch_Rev3.0:GEN_R_0201 -> R0402
- R17: value 100K -> R0402; footprint XWatch_Rev3.0:GEN_R_0201 -> R0402
- moved R14 91.6 mm to (100.0, 60.6)
- moved R21 90.8 mm to (105.1, 60.1), turned to 90 degrees
- moved R20 90.1 mm to (103.7, 60.6)
- moved R13 87.5 mm to (100.9, 64.0), turned to 90 degrees
- moved R17 85.5 mm to (94.9, 67.6), turned to -90 degrees
- moved R16 84.9 mm to (97.6, 59.6)
- moved R15 82.1 mm to (100.0, 59.6)
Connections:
- R13 pad 1: +1V8 -> 3V3_LDO_RF
- R13 pad 2: /MCU_IO/I2C5.SDA -> 3V3_LDO_ANT
- R14 pad 1: +1V8 -> N18512190
- R14 pad 2: /MCU_IO/I2C5.SCL -> N18512210
- R15 pad 1: +1V8 -> N18512190
- R15 pad 2: /MCU_IO/ALS_INT_N -> ANT_DETECT
- R16 pad 1: +1V8 -> GND_POWER
- R16 pad 2: /MCU_IO/PPG_INT_N -> N18512190
- R17 pad 1: /MCU_IO/HAPTIC_EN -> GND_POWER
- R17 pad 2: GND -> N18512158
- R20 pad 1: +1V8 -> GND_POWER
- R20 pad 2: /MCU_IO/DSI_TP_INT -> N18512260
- R21 pad 1: +1V8 -> GND_POWER
- R21 pad 2: Net-(U14-CS) -> ANT_DETECT
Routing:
- net GND_POWER: track 0.00 -> 321.8 mm, vias 0 -> 2256
- net VBAT: track 0.00 -> 311.0 mm, vias 0 -> 10
- net VIO18: track 0.00 -> 282.8 mm, vias 0 -> 8
- net AG3335_GPIO26_O: track 0.00 -> 185.5 mm, vias 0 -> 2
- net DVDD28_IO: track 0.00 -> 148.7 mm, vias 0 -> 1
- net ANT_DETECT: track 0.00 -> 143.4 mm, vias 0 -> 1
- net UART0_TX_AG3335: track 0.00 -> 137.3 mm
- net VRTC_IN: track 0.00 -> 135.0 mm, vias 0 -> 4
- net AG3335_GPIO4_O: track 0.00 -> 134.2 mm, vias 0 -> 1
- net UART0_RX_AG3335: track 0.00 -> 131.8 mm
- net USB20_DM_AG3335: track 0.00 -> 130.8 mm, vias 0 -> 2
- net USB20_DP_AG3335: track 0.00 -> 130.4 mm, vias 0 -> 2
- net AG3335_GPIO9_O: track 0.00 -> 126.4 mm, vias 0 -> 1
- net AG3335_GPIO10_O: track 0.00 -> 122.3 mm, vias 0 -> 1
- net AVDD18_TCXO: track 0.00 -> 112.8 mm, vias 0 -> 4
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- added copper zone on B.Cu, net GND_POWER
- added copper zone on F.Cu, net GND_POWER
- added copper zone on In1.Cu, net GND_POWER
- added copper zone on In2.Cu, net GND_POWER
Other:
- board size 36 x 36 mm -> 140 x 96 mm
- copper layers 2 -> 4
- rule pad_to_mask_clearance: 0 -> 0.1016
- board text added: "140.00mm"
- board text added: "96.00mm"
- board text added: "A"
- board text added: "AG3335M_EVK_V2"
- board text added: "AVDD18"
- board text added: "B"
- board text added: "C"
- board text added: "DVDD28"
- board text added: "GPIO0"
- board text added: "GPIO1"
- board text added: "GPIO10"
- board text added: "GPIO11"
- board text added: "GPIO12"
- board text added: "GPIO13"
- board text added: "GPIO14"
- board text added: "GPIO15"
- board text added: "GPIO16"
- board text added: "GPIO17"
- board text added: "GPIO18"
- board text added: "GPIO19"
- board text added: "GPIO2"
- board text added: "GPIO20"
- board text added: "GPIO21"
- board text added: "GPIO22"
- board text added: "GPIO23"
- board text added: "GPIO24"
- board text added: "GPIO25"
- board text added: "GPIO26"
- board text added: "GPIO27"
- board text added: "GPIO28"
- board text added: "GPIO29"
- board text added: "GPIO3"
- board text added: "GPIO4"
- board text added: "GPIO5"
- board text added: "GPIO6"
- board text added: "GPIO7"
- board text added: "GPIO8"
- board text added: "GPIO9"
- board text added: "VCCK"
- board text added: "VIO18"
- board text added: "VRF"
- board text added: "VRTC"
- board text added: "VSRAM"
- board text added: "[C727]"
- board text added: "_TCXO"
